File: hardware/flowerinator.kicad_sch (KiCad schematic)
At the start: 11 parts, among them J1 HY-SRF05 ultrasonic, M1 Motor_DC, Q1 Q_NMOS_GDS, Q2 Q_NMOS_GDS, U1 ESP32-WROOM-32, U2 Water sensor, U3 Height Sensor, U4 Soil Sensor, U5 Soil Sensor

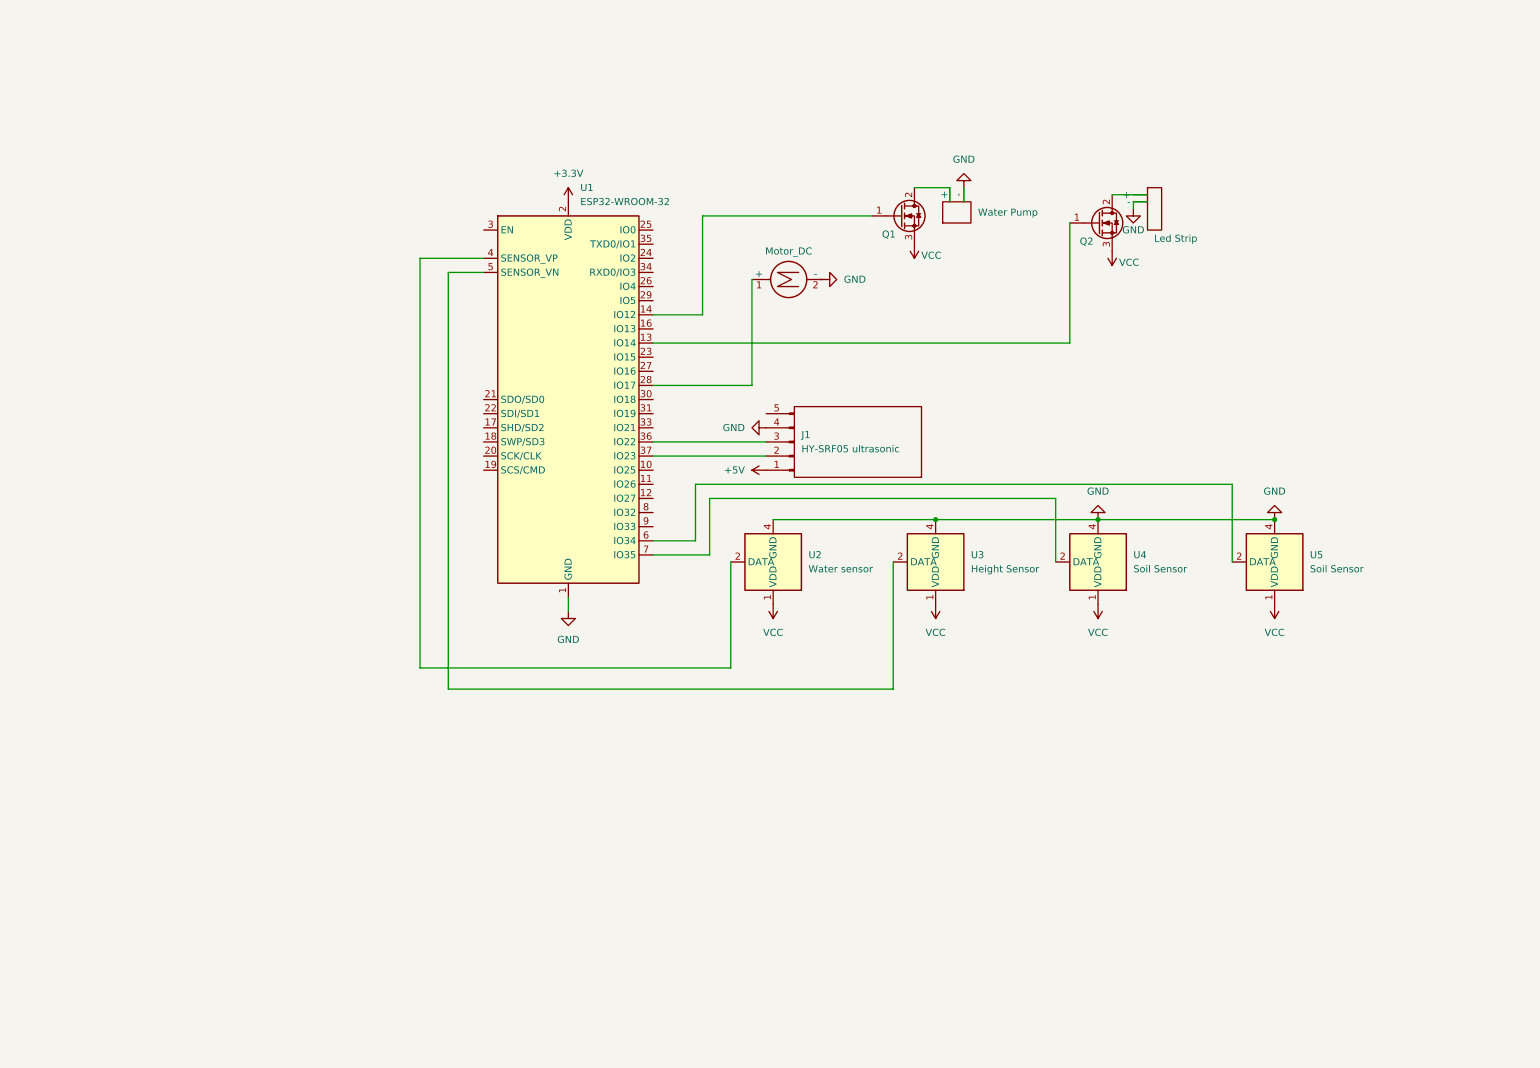
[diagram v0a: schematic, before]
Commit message: finished the pcb
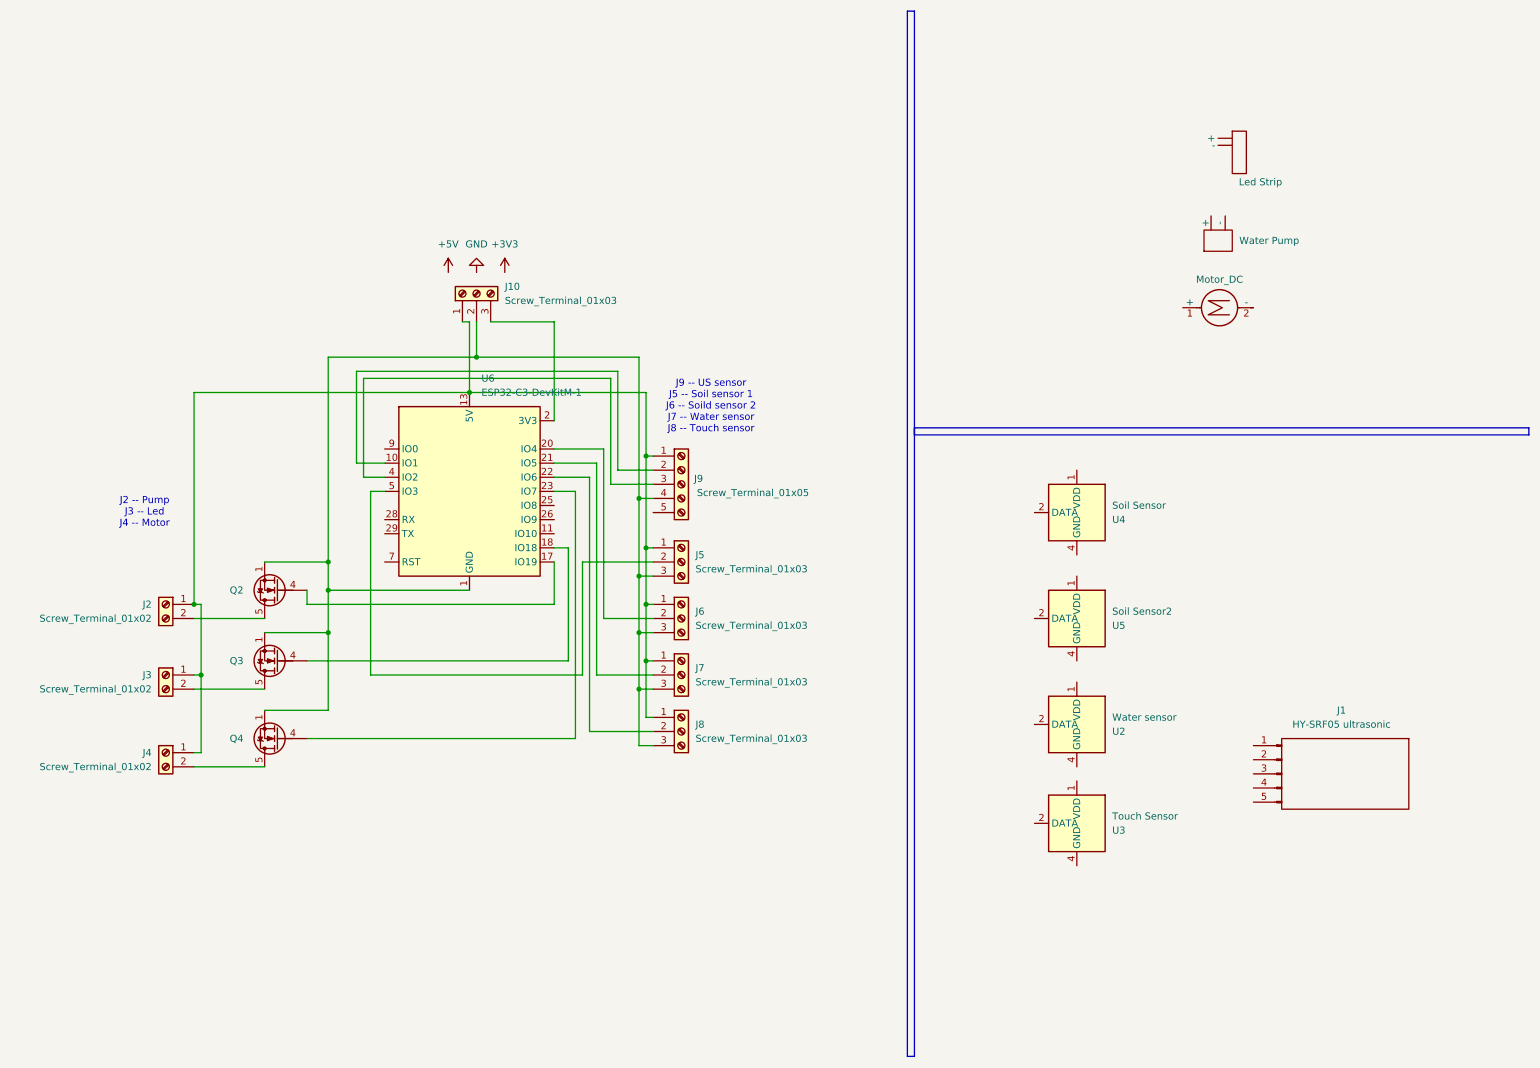
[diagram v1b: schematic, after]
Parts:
- removed Q1, Q2: Q_NMOS_GDS, symbol Transistor_FET:Q_NMOS_GDS
- removed U1: ESP32-WROOM-32, RF_Module:ESP32-WROOM-32, symbol RF_Module:ESP32-WROOM-32
- added J10, J5, J6, J7, J8: Screw_Terminal_01x03, Connector_Phoenix_GMSTB:PhoenixContact_GMSTBVA_2,5_3-G_1x03_P7.50mm_Vertical, symbol Connector:Screw_Terminal_01x03
- added J2, J4: Screw_Terminal_01x02, Connector_Phoenix_GMSTB:PhoenixContact_GMSTBVA_2,5_2-G_1x02_P7.50mm_Vertical, symbol Connector:Screw_Terminal_01x02
- added J3: Screw_Terminal_01x02, Connector_Phoenix_GMSTB:PhoenixContact_GMSTBV_2,5_2-GF-7,62_1x02_P7.62mm_Vertical_ThreadedFlange, symbol Connector:Screw_Terminal_01x02
- added J9: Screw_Terminal_01x05, Connector_Phoenix_GMSTB:PhoenixContact_GMSTBVA_2,5_5-G_1x05_P7.50mm_Vertical, symbol Connector:Screw_Terminal_01x05
- added Q2, Q3, Q4: FDMS8350LET40, Package_TO_SOT_SMD:TDSON-8-1, symbol Transistor_FET:FDMS8350LET40
- added U6: ESP32-C3-DevKitM-1, RF_Module:ESP32-C3-DevKitM-1, symbol RF_Module:ESP32-C3-DevKitM-1
- U3: value Height Sensor -> Touch Sensor
- U5: value Soil Sensor -> Soil Sensor2
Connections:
- net +5V: no longer J1.1 (Vcc)
- net GND: no longer J1.4 (GND), L1. (-), M1.2 (-), U2.4 (GND), U3.4 (GND), U4.4 (GND), U5.4 (GND), W1. (-)
- removed net VCC: U2.1 (VDD), U3.1 (VDD), U4.1 (VDD), U5.1 (VDD)
- new net: J10.2 (Pin_2), J5.3 (Pin_3), J6.3 (Pin_3), J7.3 (Pin_3), J8.3 (Pin_3), J9.4 (Pin_4), Q2.1 (S), Q2.2 (S), Q2.3 (S), Q3.1 (S), Q3.2 (S), Q3.3 (S), Q4.1 (S), Q4.2 (S), Q4.3 (S), U6.1 (GND), U6.12 (GND), U6.15 (GND), U6.16 (GND), U6.19 (GND), U6.24 (GND), U6.27 (GND), U6.30 (GND), U6.6 (GND), U6.8 (GND)
- new net: Q2.4 (G), U6.17 (IO19)
- new net: J2.2 (Pin_2), Q2.5 (D)
- new net: Q4.4 (G), U6.23 (IO7)
- new net: J4.2 (Pin_2), Q4.5 (D)
- new net: J10.1 (Pin_1), J2.1 (Pin_1), J3.1 (Pin_1), J4.1 (Pin_1), J5.1 (Pin_1), J6.1 (Pin_1), J7.1 (Pin_1), J8.1 (Pin_1), J9.1 (Pin_1), U6.13 (5V), U6.14 (5V)
- new net: J10.3 (Pin_3), U6.2 (3V3), U6.3 (3V3)
- new net: J8.2 (Pin_2), U6.22 (IO6)
- new net: Q3.4 (G), U6.18 (IO18)
- new net: J3.2 (Pin_2), Q3.5 (D)
- new net: J6.2 (Pin_2), U6.20 (IO4)
- new net: J9.2 (Pin_2), U6.10 (IO1)
- new net: J9.3 (Pin_3), U6.4 (IO2)
- new net: J7.2 (Pin_2), U6.21 (IO5)
- new net: J5.2 (Pin_2), U6.5 (IO3)
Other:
- note added: "J2 -- Pump J3 -- Led J4 -- Motor"
- note added: "J9 -- US sensor J5 -- Soil sensor 1 J6 -- Soild sensor 2 J7 -- Water sensor J8 -- Touch sensor"
- moved on the sheet: J1, U2, U3, U4, U5

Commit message: schematic
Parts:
- J3: footprint Connector_Phoenix_GMSTB:PhoenixContact_GMSTBV_2,5_2-GF-7,62_1x02_P7.62mm_Vertical_ThreadedFlange -> Connector_Phoenix_GMSTB:PhoenixContact_GMSTBVA_2,5_2-G_1x02_P7.50mm_Vertical
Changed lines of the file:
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@@
 			)
 		)
-		(property "Footprint" "Connector_Phoenix_GMSTB:PhoenixContact_GMSTBV_2,5_2-GF-7,62_1x02_P7.62mm_Vertical_ThreadedFlange"
+		(property "Footprint" "Connector_Phoenix_GMSTB:PhoenixContact_GMSTBVA_2,5_2-G_1x02_P7.50mm_Vertical"
 			(at 41.91 129.54 0)
 			(hide yes)
